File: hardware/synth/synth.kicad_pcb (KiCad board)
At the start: 2 copper layers, 20 x 50 mm, 0 parts

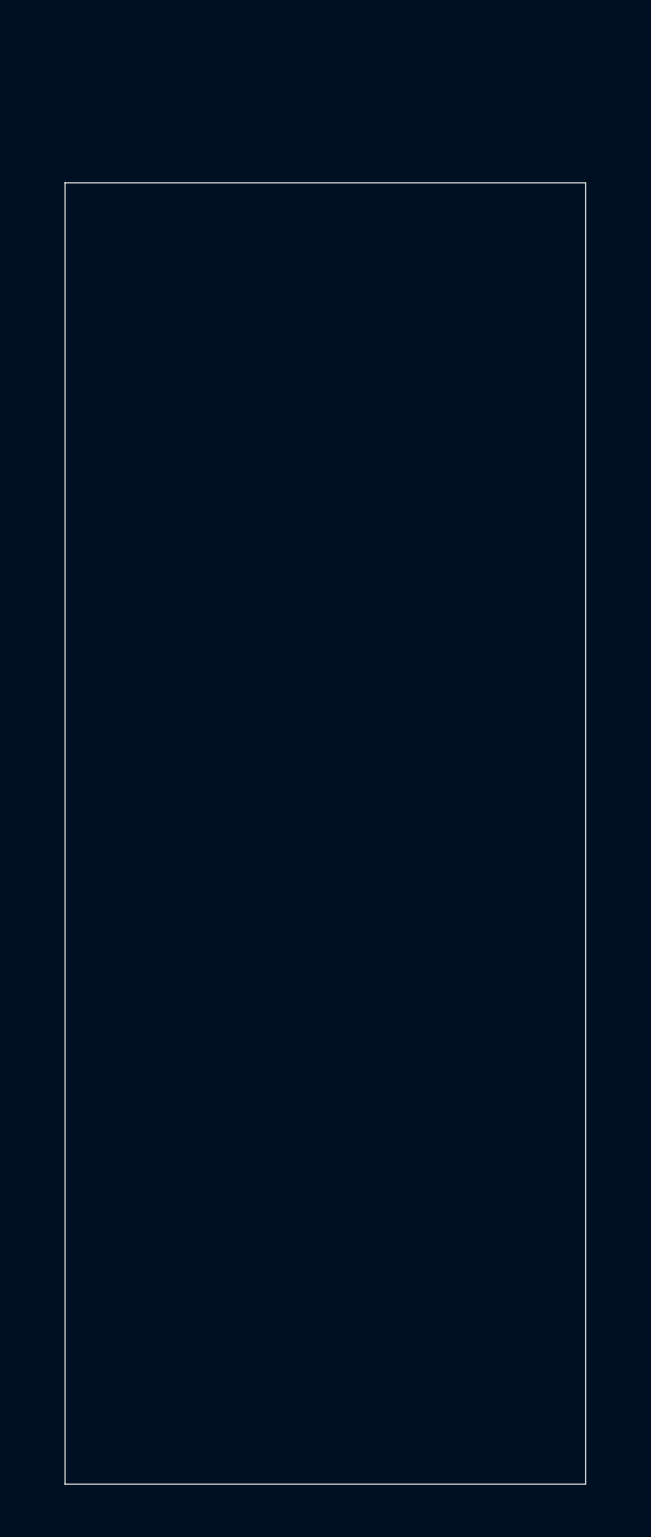
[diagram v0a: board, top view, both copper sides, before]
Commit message: Hardware rev 2 and some firmware updates
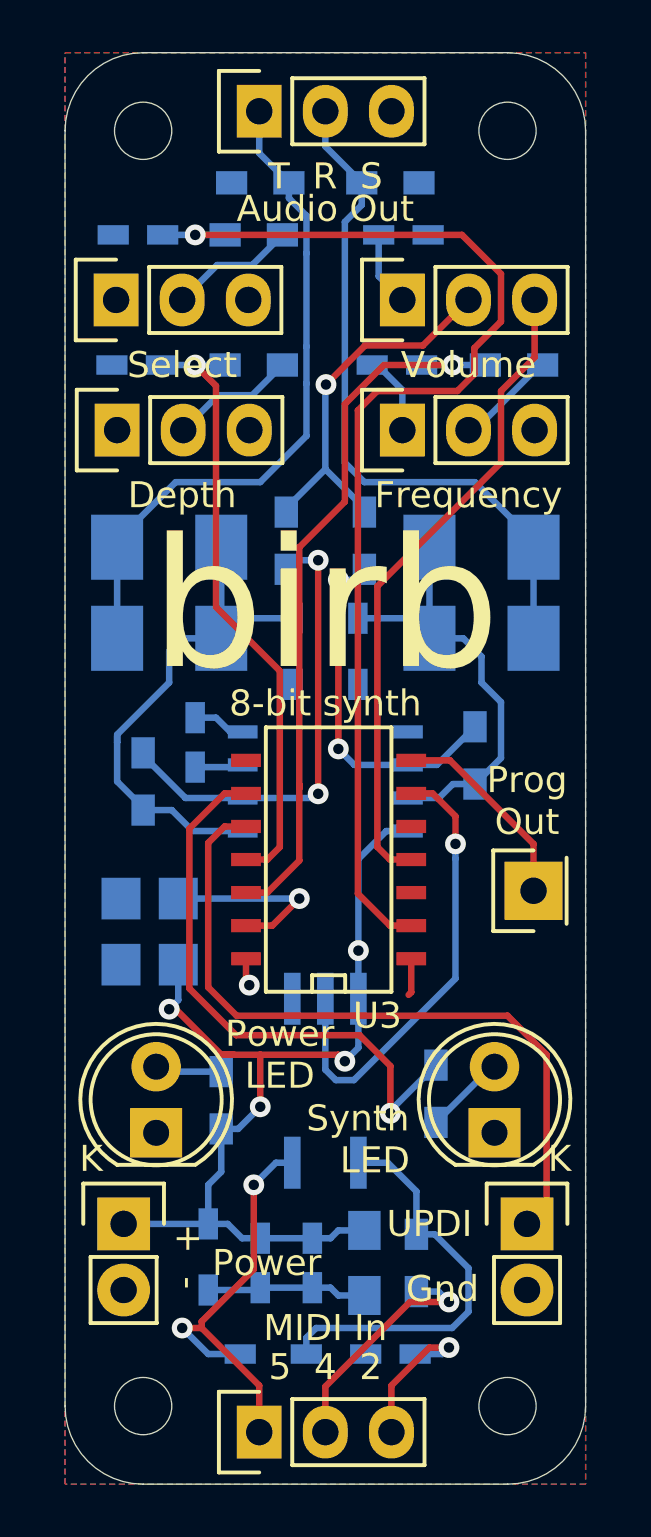
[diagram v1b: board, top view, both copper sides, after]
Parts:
- added BT1: Battery, Pin_Headers:Pin_Header_Straight_1x02, F.Cu at (122.2, 110.0)
- added C1: 10u, Capacitors_SMD:C_0805_HandSoldering, B.Cu at (131.5, 111.5)
- added C10: 47U, Capacitors_SMD:C_1210_HandSoldering, B.Cu at (136.0, 87.5)
- added C11: 100n, Capacitors_SMD:C_0603_HandSoldering, B.Cu at (122.8, 77.0)
- added C12: 100n, Capacitors_SMD:C_0603_HandSoldering, B.Cu at (132.8, 77.0)
- added C13: 100n, Capacitors_SMD:C_0603_HandSoldering, B.Cu at (122.8, 72.0)
- added C2: 100n, Capacitors_SMD:C_0603_HandSoldering, B.Cu at (127.5, 111.5)
- added C3: 1U, Capacitors_SMD:C_0603_HandSoldering, B.Cu at (133.0, 72.0)
- added C4: 1n, Capacitors_SMD:C_0603_HandSoldering, B.Cu at (129.5, 111.5)
- added C5: 1U, Capacitors_SMD:C_0603_HandSoldering, B.Cu at (125.0, 91.5)
- added C6: DNL, Capacitors_SMD:C_0603_HandSoldering, B.Cu at (132.5, 115.0)
- added C7: 47U, Capacitors_SMD:C_1210_HandSoldering, B.Cu at (124.0, 84.0)
- added C8: 47U, Capacitors_SMD:C_1210_HandSoldering, B.Cu at (124.0, 87.5)
- added C9: 47U, Capacitors_SMD:C_1210_HandSoldering, B.Cu at (136.0, 84.0)
- added D1: TVS, synth:SOD-323-handsoldering, B.Cu at (125.5, 111.3)
- added D2: POWER, LEDs:LED-5MM, F.Cu at (123.5, 106.5)
- added D3: LED, LEDs:LED-5MM, F.Cu at (136.5, 106.5)
- added D4: TVS, synth:SOD-323-handsoldering, B.Cu at (128.8, 88.0)
- added D5: TVS, synth:SOD-323-handsoldering, B.Cu at (131.2, 88.0)
- added D6: TVS, synth:SOD-323-handsoldering, B.Cu at (128.0, 115.0)
- added J1: TTL_MIDI_OUT, Pin_Headers:Pin_Header_Straight_1x01, F.Cu at (138.0, 97.2)
- added J2: MIDI In, Pin_Headers:Pin_Header_Straight_1x03, F.Cu at (127.5, 118.0)
- added J3: Audio Out, Pin_Headers:Pin_Header_Straight_1x03, F.Cu at (127.5, 67.2)
- added J4: UPDI, Pin_Headers:Pin_Header_Straight_1x02, F.Cu at (137.8, 110.0)
- added R1: 22K, Resistors_SMD:R_0603_HandSoldering, B.Cu at (128.5, 83.8)
- added R10: 100K, Resistors_SMD:R_0603_HandSoldering, B.Cu at (127.2, 77.0)
- added R11: 100K, Resistors_SMD:R_0603_HandSoldering, B.Cu at (137.2, 77.0)
- added R12: 100K, Resistors_SMD:R_0603_HandSoldering, B.Cu at (127.2, 72.0)
- added R2: 22K, Resistors_SMD:R_0603_HandSoldering, B.Cu at (131.5, 83.8)
- added R3: 220R, Resistors_SMD:R_0603_HandSoldering, B.Cu at (126.0, 105.2)
- added R4: 220R, Resistors_SMD:R_0603_HandSoldering, B.Cu at (134.2, 105.0)
- added R5: 18K, Resistors_SMD:R_0603_HandSoldering, B.Cu at (123.0, 93.0)
- added R6: 18K, Resistors_SMD:R_0603_HandSoldering, B.Cu at (135.8, 92.0)
- added R7: 220R, Resistors_SMD:R_0603_HandSoldering, B.Cu at (133.5, 111.5)
- added R8: 1M, Resistors_SMD:R_0603_HandSoldering, B.Cu at (127.5, 70.0)
- added R9: 1M, Resistors_SMD:R_0603_HandSoldering, B.Cu at (132.5, 70.0)
- added REF**: MountingHole_2.2mm_M2, Mounting_Holes:MountingHole_2.2mm_M2, F.Cu at (123.0, 117.0)
- added REF**: MountingHole_2.2mm_M2, Mounting_Holes:MountingHole_2.2mm_M2, F.Cu at (123.0, 68.0)
- added REF**: MountingHole_2.2mm_M2, Mounting_Holes:MountingHole_2.2mm_M2, F.Cu at (137.0, 68.0)
- added REF**: MountingHole_2.2mm_M2, Mounting_Holes:MountingHole_2.2mm_M2, F.Cu at (137.0, 117.0)
- added RV1: 50K LOG, Pin_Headers:Pin_Header_Straight_1x03, F.Cu at (133.0, 74.5)
- added RV2: 50K LIN, Pin_Headers:Pin_Header_Straight_1x03, F.Cu at (122.0, 79.5)
- added RV3: 50K LIN, Pin_Headers:Pin_Header_Straight_1x03, F.Cu at (133.0, 79.5)
- added RV4: 50K LIN, Pin_Headers:Pin_Header_Straight_1x03, F.Cu at (122.0, 74.5)
- added U1: TPA6111A2, SMD_Packages:SOIC-8-N, B.Cu at (130.0, 93.0)
- added U2: TLP2312, Package_SO:SO-6_4.4x3.6mm_P1.27mm, B.Cu at (130.0, 104.5)
- added U3: ATtiny1614-SS, SMD_Packages:SOIC-14_N, F.Cu at (130.0, 96.0)
- added X1: DSC1001, synth:DSC_1001_Oscillator_SMD_5032_4Pads, B.Cu at (123.2, 98.8)
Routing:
- net /SELECT: track 0.00 -> 45.2 mm, vias 0 -> 1
- net VDD: track 0.00 -> 39.0 mm, vias 0 -> 4
- net /FREQ: track 0.00 -> 28.2 mm, vias 0 -> 1
- net /UPDI: track 0.00 -> 28.1 mm
- net Net-(C10-Pad1): track 0.00 -> 27.1 mm
- net Net-(C7-Pad1): track 0.00 -> 26.2 mm
- net /DAC: track 0.00 -> 25.0 mm
- net /DEPTH: track 0.00 -> 23.8 mm, vias 0 -> 1
- net /LED: track 0.00 -> 22.2 mm, vias 0 -> 1
- net Net-(C7-Pad2): track 0.00 -> 21.0 mm
- net Net-(R1-Pad1): track 0.00 -> 17.9 mm, vias 0 -> 2
- net /MIDI_IN: track 0.00 -> 17.8 mm, vias 0 -> 1
- net Net-(C10-Pad2): track 0.00 -> 17.5 mm
- net Net-(D6-Pad2): track 0.00 -> 16.5 mm, vias 0 -> 2
- net Net-(D6-Pad1): track 0.00 -> 15.8 mm
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- added copper zone on B.Cu, net GND
- added copper zone on F.Cu, net VDD
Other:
- board size 20 x 50 mm -> 20 x 55 mm
- net class Default removed
- board text added: "+ -"
- board text added: "5 4 2"
- board text added: "8-bit synth"
- board text added: "Audio Out"
- board text added: "Depth"
- board text added: "Frequency"
- board text added: "Gnd"
- board text added: "MIDI In"
- board text added: "Power"
- board text added: "Power LED"
- board text added: "Prog Out"
- board text added: "Select"
- board text added: "Synth LED"
- board text added: "T R S"
- board text added: "UPDI"
- board text added: "Volume"
- board text added: "birb"
- board text added: "rev 2 by Eric Van Albert"
